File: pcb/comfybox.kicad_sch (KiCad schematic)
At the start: 26 parts, among them K1 SW_CHOC, K2 SW_CHOC, K3 SW_CHOC, K4 SW_CHOC, P1 SW_CHOC, P2 SW_CHOC, P3 SW_CHOC, P4 SW_CHOC

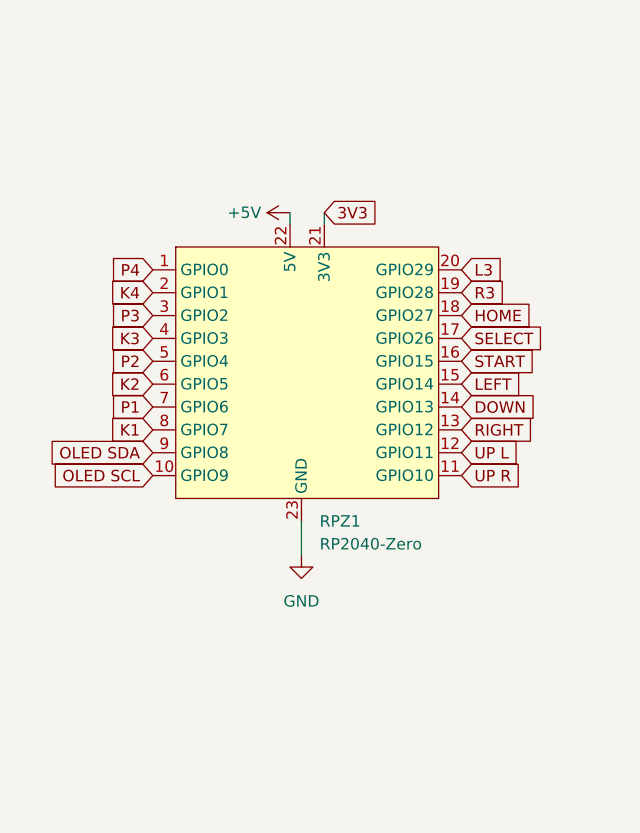
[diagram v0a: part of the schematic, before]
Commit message: pcb changes
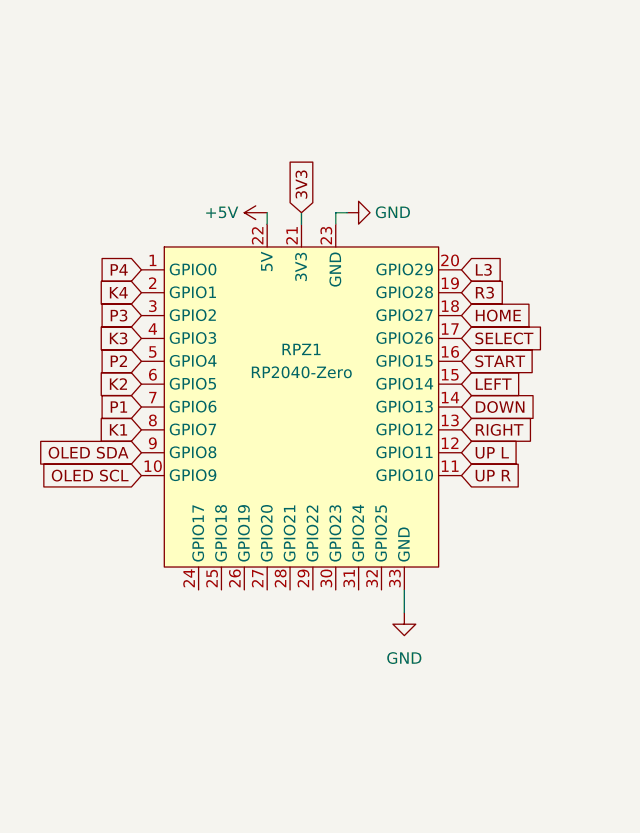
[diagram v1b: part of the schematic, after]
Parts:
- removed RPZ1: RP2040-Zero, RP2040-Zero:RP2040-Zero_reversible, symbol RP2040-Zero:RP2040-Zero
- added RPZ1: RP2040-Zero, RP2040-Zero:RP2040-Zero_reversible_extra, symbol RP2040-Zero:RP2040-Zero-Extra
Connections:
- net +5V: now also RPZ1.22 (5V)
- net 3V3: now also RPZ1.21 (3V3)
- net DOWN: now also RPZ1.14 (GPIO13)
- net GND: now also RPZ1.23 (GND), RPZ1.33 (GND)
- net HOME: now also RPZ1.18 (GPIO27)
- net K1: now also RPZ1.8 (GPIO7)
- net K2: now also RPZ1.6 (GPIO5)
- net K3: now also RPZ1.4 (GPIO3)
- net K4: now also RPZ1.2 (GPIO1)
- net L3: now also RPZ1.20 (GPIO29)
- net LEFT: now also RPZ1.15 (GPIO14)
- net OLED SCL: now also RPZ1.10 (GPIO9)
- net OLED SDA: now also RPZ1.9 (GPIO8)
- net P1: now also RPZ1.7 (GPIO6)
- net P2: now also RPZ1.5 (GPIO4)
- net P3: now also RPZ1.3 (GPIO2)
- net P4: now also RPZ1.1 (GPIO0)
- net R3: now also RPZ1.19 (GPIO28)
- net RIGHT: now also RPZ1.13 (GPIO12)
- net SELECT: now also RPZ1.17 (GPIO26)
- net START: now also RPZ1.16 (GPIO15)
- net UP L: now also RPZ1.12 (GPIO11)
- net UP R: now also RPZ1.11 (GPIO10)
